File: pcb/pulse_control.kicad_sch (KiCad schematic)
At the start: 1 part

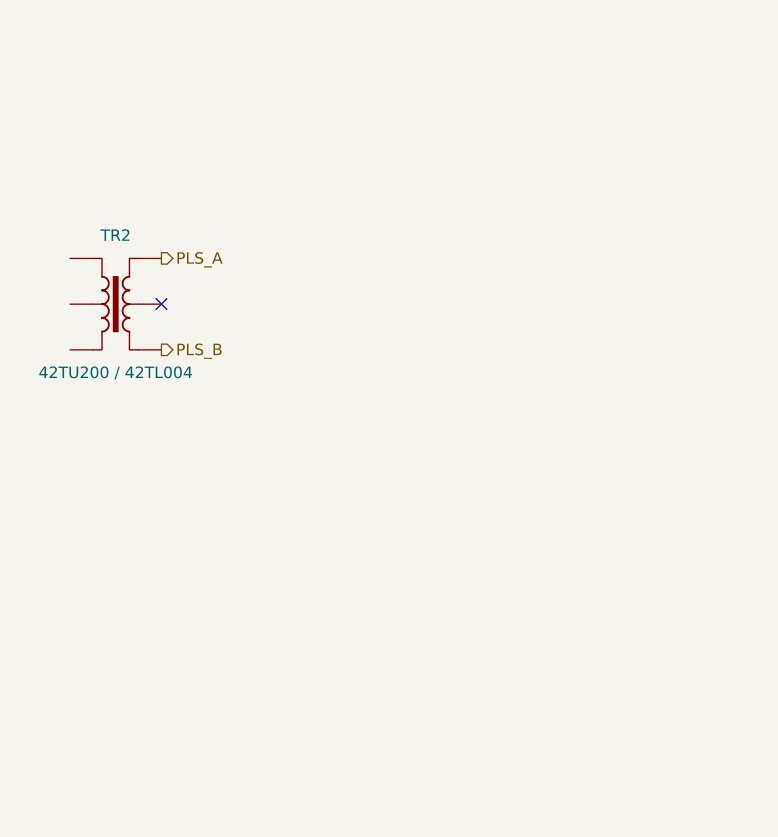
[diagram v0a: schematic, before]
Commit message: WiP level control
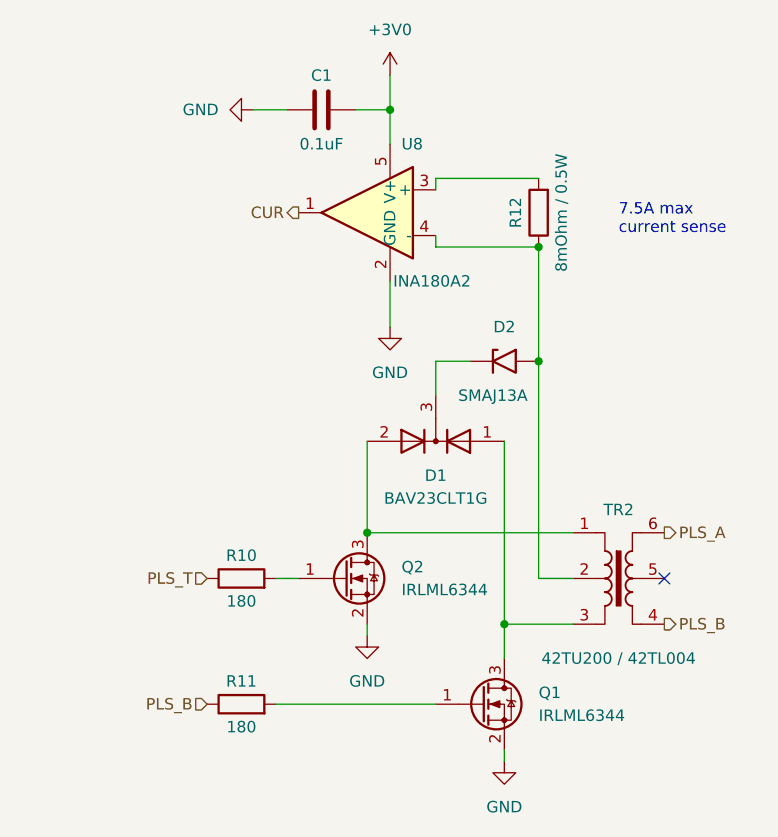
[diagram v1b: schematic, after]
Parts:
- added C1: 0.1uF, symbol Device:C
- added D1: BAV23CLT1G, symbol Diode:BAV70
- added D2: SMAJ13A, Diode_SMD:D_SMA, symbol Diode:SMAJ13A
- added Q1, Q2: IRLML6344, symbol Device:Q_NMOS_GSD
- added R10, R11: 180, symbol Device:R
- added R12: 8mOhm / 0.5W, symbol Device:R
- added U8: INA180A2, Package_TO_SOT_SMD:SOT-23-5, symbol Amplifier_Current:INA180A2
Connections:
- net PLS_B: now also R11.1
- net at TR2.1: now also D1.2 (A), Q2.3 (D)
- net at TR2.2: now also D2.2 (A2), R12.1, U8.4 (-)
- net at TR2.3: now also D1.1 (A), Q1.3 (D)
- new net: D1.3 (K), D2.1 (A1)
- new net: Q2.1 (G), R10.2
- new net: Q1.1 (G), R11.2
- new net: R12.2, U8.3 (+)
- new net +3V0: C1.1, U8.5 (V+)
- new net CUR: U8.1
- new net GND: C1.2, Q1.2 (S), Q2.2 (S), U8.2 (GND)
- new net PLS_T: R10.1
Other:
- note added: "7.5A max current sense"
